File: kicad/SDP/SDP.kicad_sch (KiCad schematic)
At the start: 84 parts, among them J1 GPIO, J2 SPI, J24 POWER, J25 Conn_01x04, J26 Conn_01x02, J27 MOTOR, J3 UART, J4 I2C, J5 Conn_01x04, J6 Conn_01x04, J7 RJ25, SW1 SW_Push_Dual, U1 TPS54233, U2 TPS54233, U3 PIC24FJ128GA010-I/PT, U4 DS3231SN-T&R, Y1 8MHz, Y2 32.768kHz

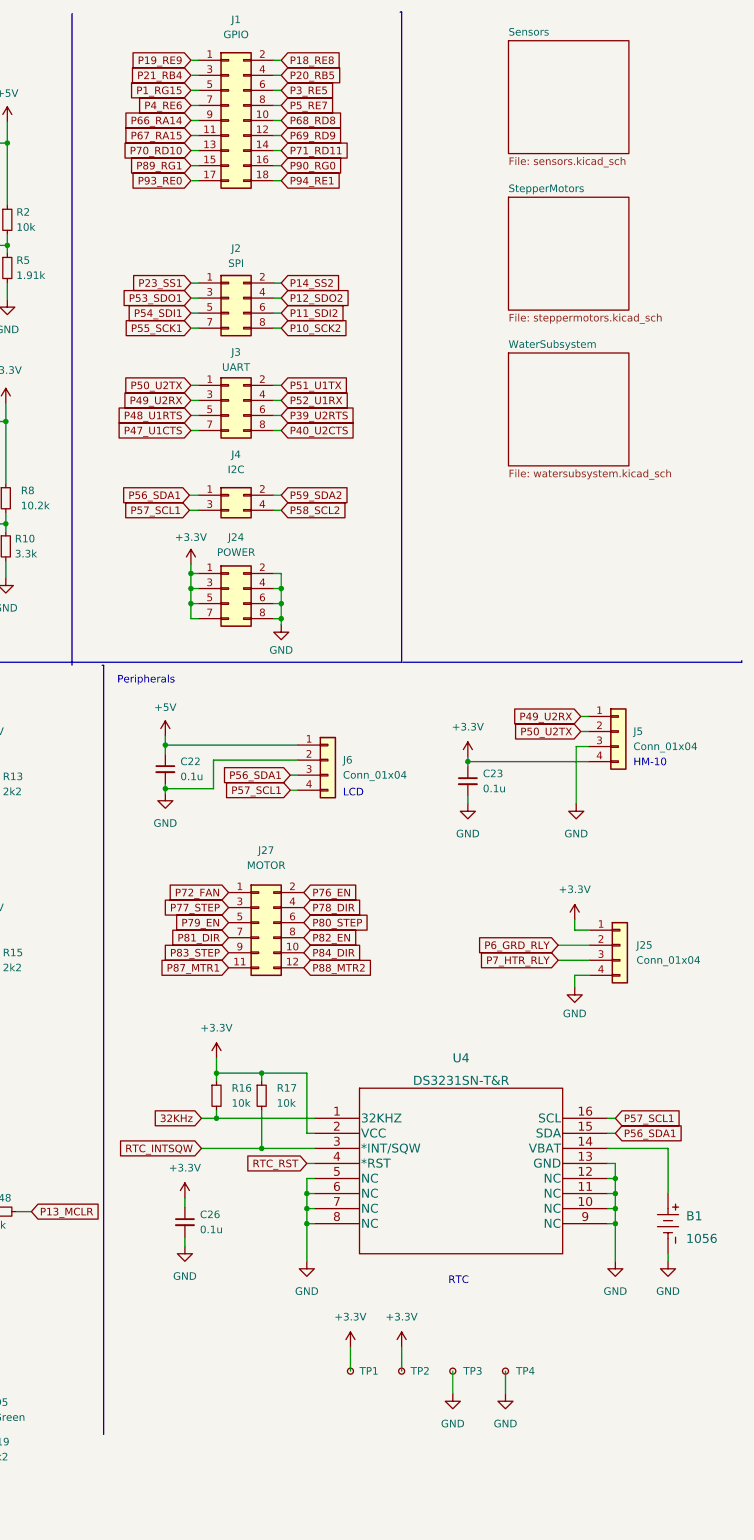
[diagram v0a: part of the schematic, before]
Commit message: PCB layout of main controller board
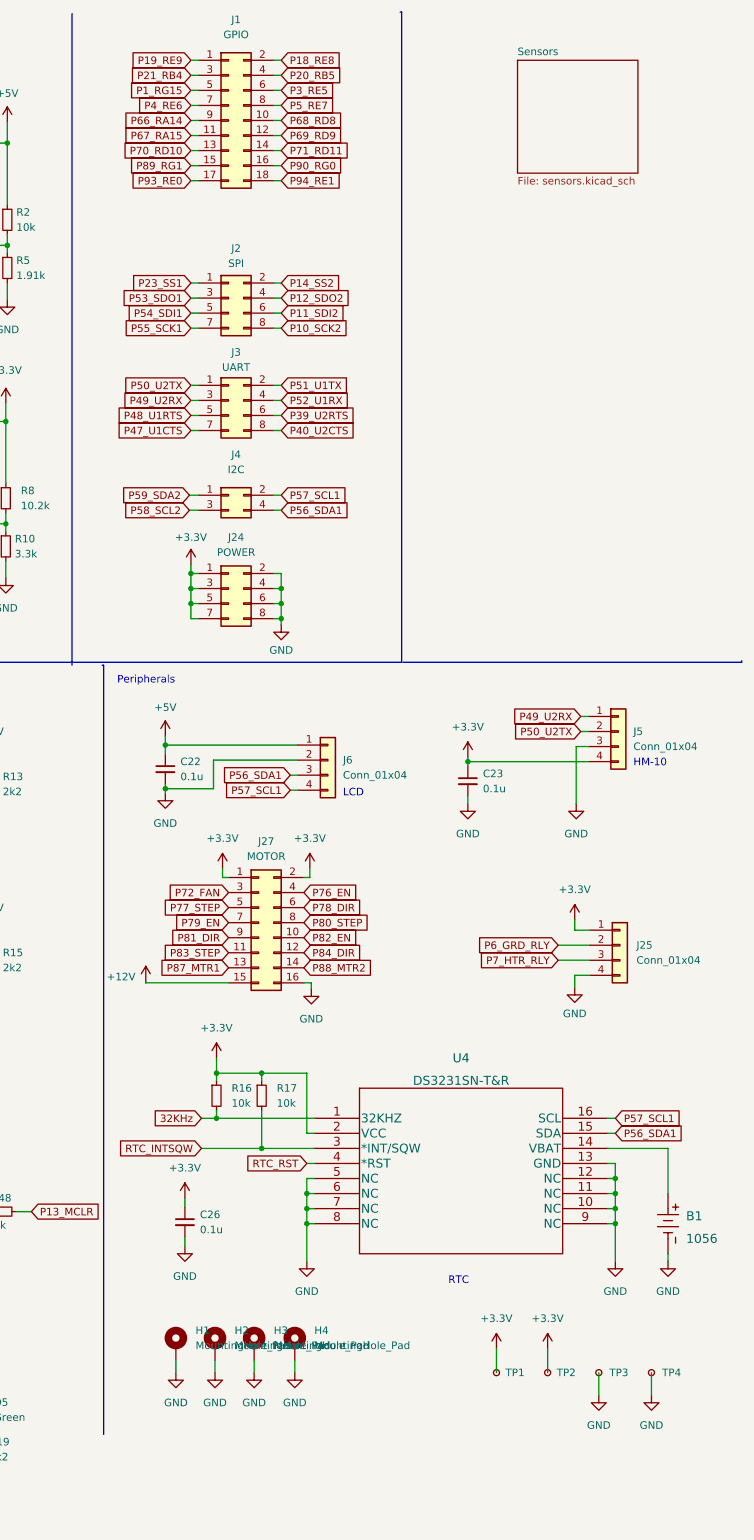
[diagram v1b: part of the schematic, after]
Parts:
- removed J27: MOTOR, Connector_PinSocket_2.54mm:PinSocket_2x04_P2.54mm_Vertical, symbol Connector_Generic:Conn_02x06_Odd_Even
- added H1, H2, H3, H4: MountingHole_Pad, MountingHole:MountingHole_3.2mm_M3_Pad, symbol Mechanical:MountingHole_Pad
- added J27: MOTOR, Connector_PinSocket_2.54mm:PinSocket_2x08_P2.54mm_Vertical, symbol Connector_Generic:Conn_02x08_Odd_Even
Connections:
- net +12V: now also J27.15 (Pin_15)
- net +3V3: now also J27.1 (Pin_1), J27.2 (Pin_2)
- net GND: now also H1.1, H2.1, H3.1, H4.1, J27.16 (Pin_16)
- net P56_SDA1: now also J4.4 (Pin_4); no longer J4.1 (Pin_1)
- net P57_SCL1: now also J4.2 (Pin_2); no longer J4.3 (Pin_3)
- net P58_SCL2: now also J4.3 (Pin_3); no longer J4.4 (Pin_4)
- net P59_SDA2: now also J4.1 (Pin_1); no longer J4.2 (Pin_2)
- net P72_FAN: now also J27.3 (Pin_3)
- net P76_EN: now also J27.4 (Pin_4)
- net P77_STEP: now also J27.5 (Pin_5)
- net P78_DIR: now also J27.6 (Pin_6)
- net P79_EN: now also J27.7 (Pin_7)
- net P80_STEP: now also J27.8 (Pin_8)
- net P81_DIR: now also J27.9 (Pin_9)
- net P82_EN: now also J27.10 (Pin_10)
- net P83_STEP: now also J27.11 (Pin_11)
- net P84_DIR: now also J27.12 (Pin_12)
- net P87_MTR1: now also J27.13 (Pin_13)
- net P88_MTR2: now also J27.14 (Pin_14)
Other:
- removed sheet StepperMotors
- removed sheet WaterSubsystem
- moved on the sheet: TP1, TP2, TP3, TP4

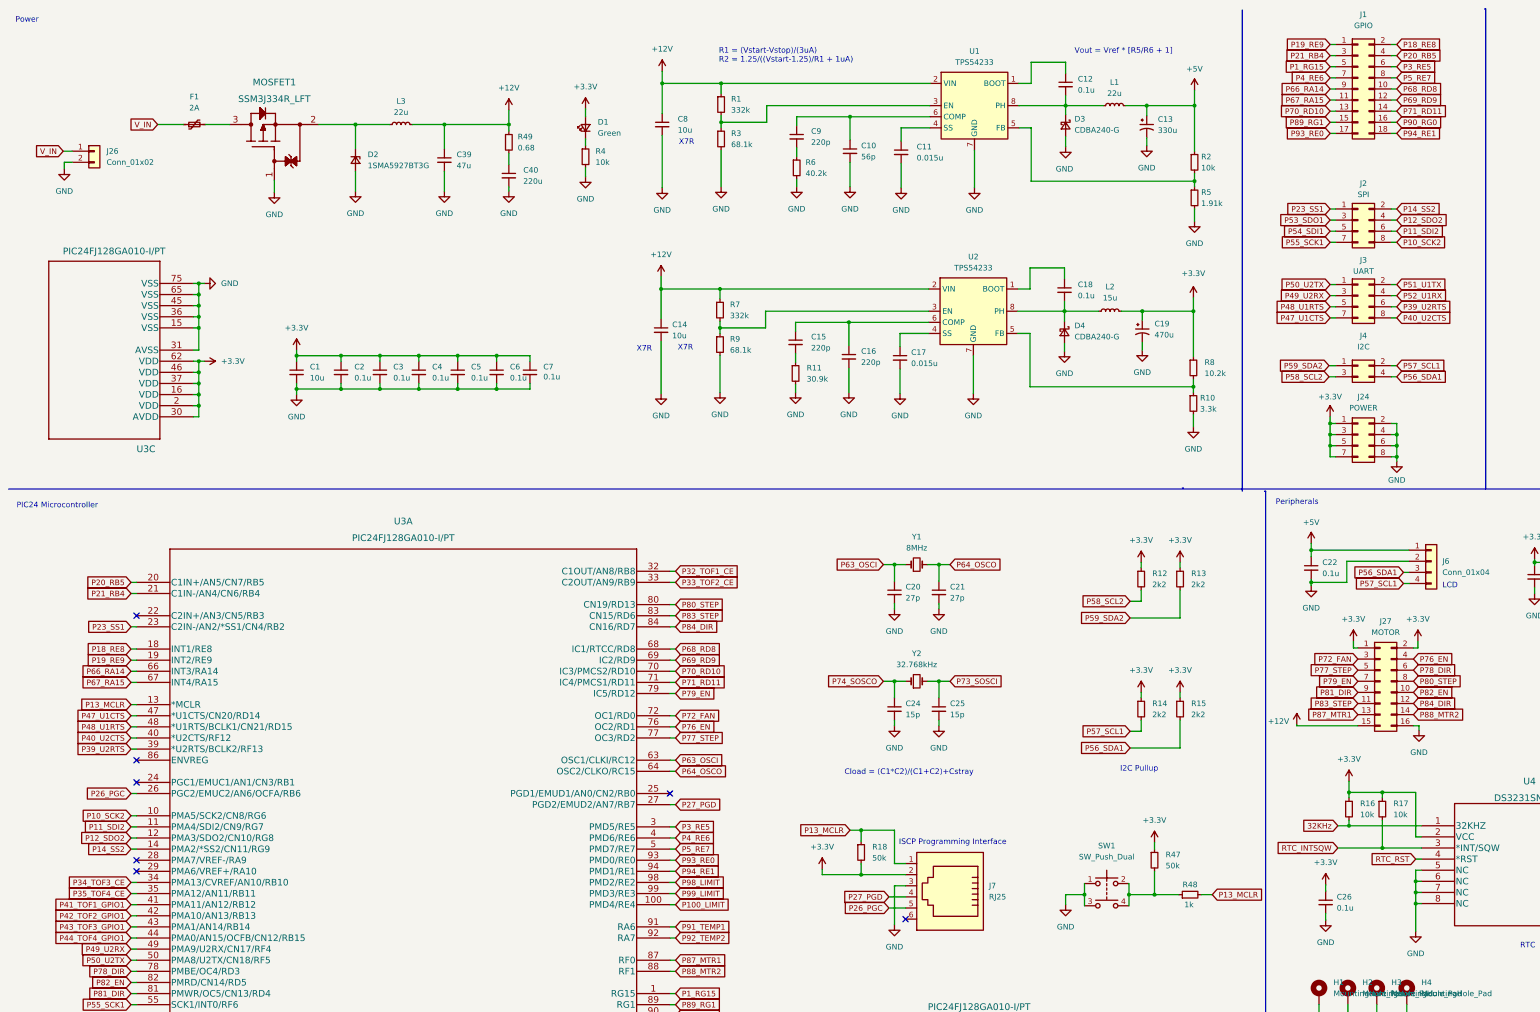
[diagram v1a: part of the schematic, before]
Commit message: Controller PCB layout
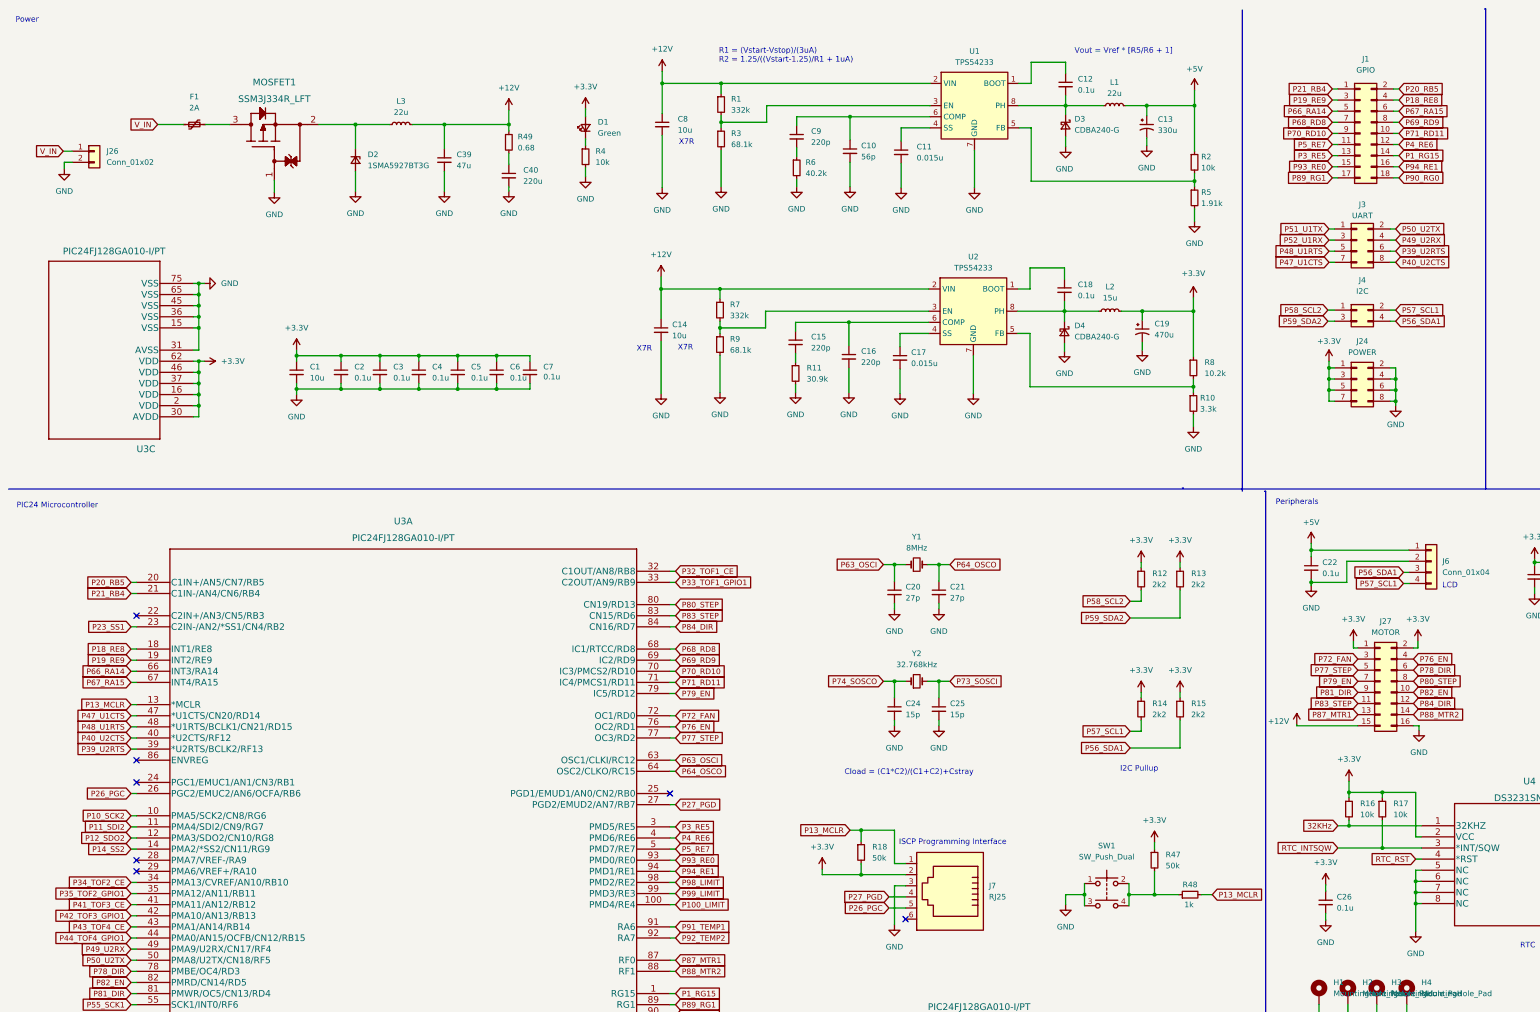
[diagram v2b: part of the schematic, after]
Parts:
- removed J2: SPI, Connector_PinSocket_2.54mm:PinSocket_2x04_P2.54mm_Vertical, symbol Connector_Generic:Conn_02x04_Odd_Even
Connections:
- net P18_RE8: now also J1.4 (Pin_4); no longer J1.2 (Pin_2)
- net P19_RE9: now also J1.3 (Pin_3); no longer J1.1 (Pin_1)
- net P1_RG15: now also J1.14 (Pin_14); no longer J1.5 (Pin_5)
- net P20_RB5: now also J1.2 (Pin_2); no longer J1.4 (Pin_4)
- net P21_RB4: now also J1.1 (Pin_1); no longer J1.3 (Pin_3)
- net P3_RE5: now also J1.13 (Pin_13); no longer J1.6 (Pin_6)
- net P49_U2RX: now also J3.4 (Pin_4); no longer J3.3 (Pin_3)
- net P4_RE6: now also J1.12 (Pin_12); no longer J1.7 (Pin_7)
- net P50_U2TX: now also J3.2 (Pin_2); no longer J3.1 (Pin_1)
- net P51_U1TX: now also J3.1 (Pin_1); no longer J3.2 (Pin_2)
- net P52_U1RX: now also J3.3 (Pin_3); no longer J3.4 (Pin_4)
- net P58_SCL2: now also J4.1 (Pin_1); no longer J4.3 (Pin_3)
- net P59_SDA2: now also J4.3 (Pin_3); no longer J4.1 (Pin_1)
- net P5_RE7: now also J1.11 (Pin_11); no longer J1.8 (Pin_8)
- net P66_RA14: now also J1.5 (Pin_5); no longer J1.9 (Pin_9)
- net P67_RA15: now also J1.6 (Pin_6); no longer J1.11 (Pin_11)
- net P68_RD8: now also J1.7 (Pin_7); no longer J1.10 (Pin_10)
- net P69_RD9: now also J1.8 (Pin_8); no longer J1.12 (Pin_12)
- net P70_RD10: now also J1.9 (Pin_9); no longer J1.13 (Pin_13)
- net P71_RD11: now also J1.10 (Pin_10); no longer J1.14 (Pin_14)
- net P89_RG1: now also J1.17 (Pin_17); no longer J1.15 (Pin_15)
- net P90_RG0: now also J1.18 (Pin_18); no longer J1.16 (Pin_16)
- net P93_RE0: now also J1.15 (Pin_15); no longer J1.17 (Pin_17)
- net P94_RE1: now also J1.16 (Pin_16); no longer J1.18 (Pin_18)
- net P33_TOF2_CE renamed P33_TOF1_GPIO1
- net P34_TOF3_CE renamed P34_TOF2_CE
- net P35_TOF4_CE renamed P35_TOF2_GPIO1
- net P41_TOF1_GPIO1 renamed P41_TOF3_CE
- net P42_TOF2_GPIO1 renamed P42_TOF3_GPIO1
- net P43_TOF3_GPIO1 renamed P43_TOF4_CE
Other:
- moved on the sheet: J1, J24, J3, J4
